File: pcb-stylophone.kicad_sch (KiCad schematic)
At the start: 2 parts, among them J1 Conn_01x02_Pin, U1 NA555P

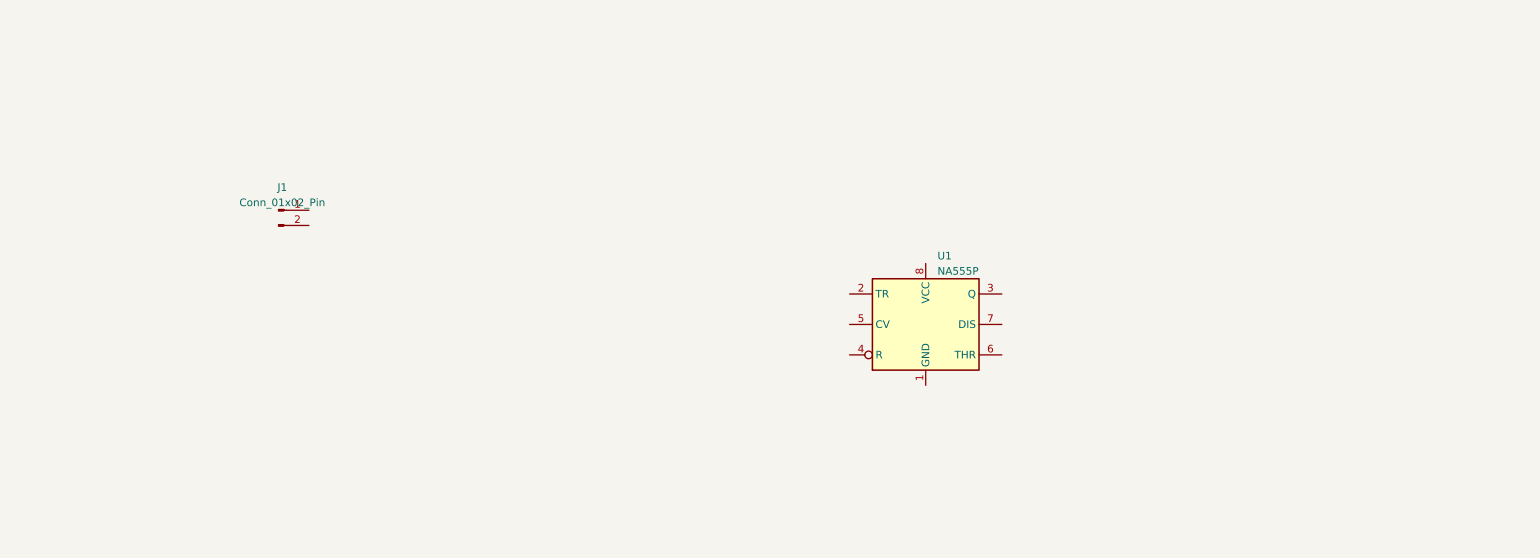
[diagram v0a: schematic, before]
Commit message: finalised v1
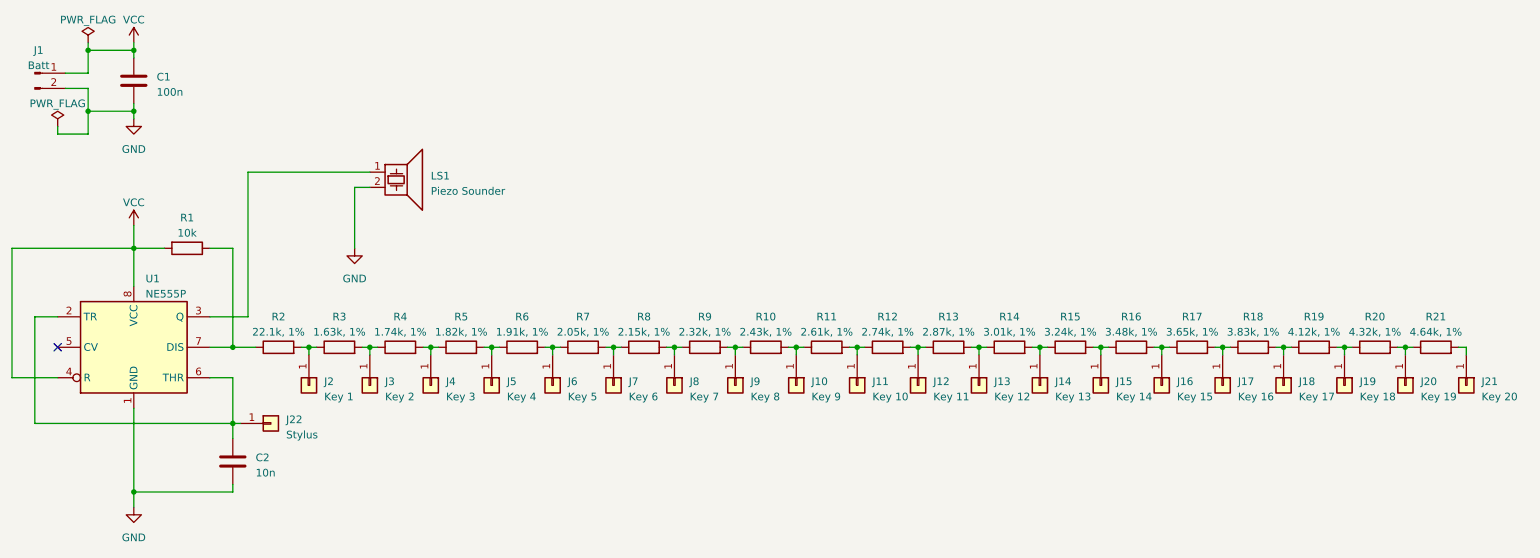
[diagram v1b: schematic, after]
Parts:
- removed U1: NA555P, Package_DIP:DIP-8_W7.62mm, symbol Timer:NA555P
- added C1: 100n, Capacitor_THT:C_Disc_D4.3mm_W1.9mm_P5.00mm, symbol Device:C
- added C2: 10n, Capacitor_THT:C_Disc_D4.3mm_W1.9mm_P5.00mm, symbol Device:C
- added J10: Key 9, TestPoint:TestPoint_Pad_1.0x1.0mm, symbol Connector_Generic:Conn_01x01
- added J11: Key 10, TestPoint:TestPoint_Pad_1.0x1.0mm, symbol Connector_Generic:Conn_01x01
- added J12: Key 11, TestPoint:TestPoint_Pad_1.0x1.0mm, symbol Connector_Generic:Conn_01x01
- added J13: Key 12, TestPoint:TestPoint_Pad_1.0x1.0mm, symbol Connector_Generic:Conn_01x01
- added J14: Key 13, TestPoint:TestPoint_Pad_1.0x1.0mm, symbol Connector_Generic:Conn_01x01
- added J15: Key 14, TestPoint:TestPoint_Pad_1.0x1.0mm, symbol Connector_Generic:Conn_01x01
- added J16: Key 15, TestPoint:TestPoint_Pad_1.0x1.0mm, symbol Connector_Generic:Conn_01x01
- added J17: Key 16, TestPoint:TestPoint_Pad_1.0x1.0mm, symbol Connector_Generic:Conn_01x01
- added J18: Key 17, TestPoint:TestPoint_Pad_1.0x1.0mm, symbol Connector_Generic:Conn_01x01
- added J19: Key 18, TestPoint:TestPoint_Pad_1.0x1.0mm, symbol Connector_Generic:Conn_01x01
- added J2: Key 1, TestPoint:TestPoint_Pad_1.0x1.0mm, symbol Connector_Generic:Conn_01x01
- added J20: Key 19, TestPoint:TestPoint_Pad_1.0x1.0mm, symbol Connector_Generic:Conn_01x01
- added J21: Key 20, TestPoint:TestPoint_Pad_1.0x1.0mm, symbol Connector_Generic:Conn_01x01
- added J22: Stylus, TestPoint:TestPoint_THTPad_D2.5mm_Drill1.2mm, symbol Connector_Generic:Conn_01x01
- added J3: Key 2, TestPoint:TestPoint_Pad_1.0x1.0mm, symbol Connector_Generic:Conn_01x01
- added J4: Key 3, TestPoint:TestPoint_Pad_1.0x1.0mm, symbol Connector_Generic:Conn_01x01
- added J5: Key 4, TestPoint:TestPoint_Pad_1.0x1.0mm, symbol Connector_Generic:Conn_01x01
- added J6: Key 5, TestPoint:TestPoint_Pad_1.0x1.0mm, symbol Connector_Generic:Conn_01x01
- added J7: Key 6, TestPoint:TestPoint_Pad_1.0x1.0mm, symbol Connector_Generic:Conn_01x01
- added J8: Key 7, TestPoint:TestPoint_Pad_1.0x1.0mm, symbol Connector_Generic:Conn_01x01
- added J9: Key 8, TestPoint:TestPoint_Pad_1.0x1.0mm, symbol Connector_Generic:Conn_01x01
- added LS1: Piezo Sounder, Buzzer_Beeper:Buzzer_D14mm_H7mm_P10mm, symbol Device:Speaker_Crystal
- added R1: 10k, Resistor_THT:R_Axial_DIN0207_L6.3mm_D2.5mm_P7.62mm_Horizontal, symbol Device:R
- added R10: 2.43k, 1%, Resistor_THT:R_Axial_DIN0207_L6.3mm_D2.5mm_P7.62mm_Horizontal, symbol Device:R
- added R11: 2.61k, 1%, Resistor_THT:R_Axial_DIN0207_L6.3mm_D2.5mm_P7.62mm_Horizontal, symbol Device:R
- added R12: 2.74k, 1%, Resistor_THT:R_Axial_DIN0207_L6.3mm_D2.5mm_P7.62mm_Horizontal, symbol Device:R
- added R13: 2.87k, 1%, Resistor_THT:R_Axial_DIN0207_L6.3mm_D2.5mm_P7.62mm_Horizontal, symbol Device:R
- added R14: 3.01k, 1%, Resistor_THT:R_Axial_DIN0207_L6.3mm_D2.5mm_P7.62mm_Horizontal, symbol Device:R
- added R15: 3.24k, 1%, Resistor_THT:R_Axial_DIN0207_L6.3mm_D2.5mm_P7.62mm_Horizontal, symbol Device:R
- added R16: 3.48k, 1%, Resistor_THT:R_Axial_DIN0207_L6.3mm_D2.5mm_P7.62mm_Horizontal, symbol Device:R
- added R17: 3.65k, 1%, Resistor_THT:R_Axial_DIN0207_L6.3mm_D2.5mm_P7.62mm_Horizontal, symbol Device:R
- added R18: 3.83k, 1%, Resistor_THT:R_Axial_DIN0207_L6.3mm_D2.5mm_P7.62mm_Horizontal, symbol Device:R
- added R19: 4.12k, 1%, Resistor_THT:R_Axial_DIN0207_L6.3mm_D2.5mm_P7.62mm_Horizontal, symbol Device:R
- added R2: 22.1k, 1%, Resistor_THT:R_Axial_DIN0207_L6.3mm_D2.5mm_P7.62mm_Horizontal, symbol Device:R
- added R20: 4.32k, 1%, Resistor_THT:R_Axial_DIN0207_L6.3mm_D2.5mm_P7.62mm_Horizontal, symbol Device:R
- added R21: 4.64k, 1%, Resistor_THT:R_Axial_DIN0207_L6.3mm_D2.5mm_P7.62mm_Horizontal, symbol Device:R
- added R3: 1.63k, 1%, Resistor_THT:R_Axial_DIN0207_L6.3mm_D2.5mm_P7.62mm_Horizontal, symbol Device:R
- added R4: 1.74k, 1%, Resistor_THT:R_Axial_DIN0207_L6.3mm_D2.5mm_P7.62mm_Horizontal, symbol Device:R
- added R5: 1.82k, 1%, Resistor_THT:R_Axial_DIN0207_L6.3mm_D2.5mm_P7.62mm_Horizontal, symbol Device:R
- added R6: 1.91k, 1%, Resistor_THT:R_Axial_DIN0207_L6.3mm_D2.5mm_P7.62mm_Horizontal, symbol Device:R
- added R7: 2.05k, 1%, Resistor_THT:R_Axial_DIN0207_L6.3mm_D2.5mm_P7.62mm_Horizontal, symbol Device:R
- added R8: 2.15k, 1%, Resistor_THT:R_Axial_DIN0207_L6.3mm_D2.5mm_P7.62mm_Horizontal, symbol Device:R
- added R9: 2.32k, 1%, Resistor_THT:R_Axial_DIN0207_L6.3mm_D2.5mm_P7.62mm_Horizontal, symbol Device:R
- added U1: NE555P, Package_DIP:DIP-8_W7.62mm, symbol Timer:NE555P
- J1: value Conn_01x02_Pin -> Batt; footprint (none) -> Connector_PinHeader_2.54mm:PinHeader_1x02_P2.54mm_Vertical
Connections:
- net VCC: now reaches J1.1 (Pin_1)
- net VCC: now also C1.1, R1.2, U1.4 (R), U1.8 (VCC)
- net GND: now reaches J1.2 (Pin_2)
- net GND: now also C1.2, C2.2, LS1.2, U1.1 (GND)
- new net: J11.1 (Pin_1), R11.2, R12.1
- new net: J12.1 (Pin_1), R12.2, R13.1
- new net: J10.1 (Pin_1), R10.2, R11.1
- new net: J21.1 (Pin_1), R21.2
- new net: R1.1, R2.1, U1.7 (DIS)
- new net: J9.1 (Pin_1), R10.1, R9.2
- new net: J17.1 (Pin_1), R17.2, R18.1
- new net: J18.1 (Pin_1), R18.2, R19.1
- new net: C2.1, J22.1 (Pin_1), U1.2 (TR), U1.6 (THR)
- new net: J15.1 (Pin_1), R15.2, R16.1
- new net: J16.1 (Pin_1), R16.2, R17.1
- new net: J20.1 (Pin_1), R20.2, R21.1
- new net: J7.1 (Pin_1), R7.2, R8.1
- new net: J8.1 (Pin_1), R8.2, R9.1
- new net: J13.1 (Pin_1), R13.2, R14.1
- new net: J14.1 (Pin_1), R14.2, R15.1
- new net: J5.1 (Pin_1), R5.2, R6.1
- new net: J4.1 (Pin_1), R4.2, R5.1
- new net: J6.1 (Pin_1), R6.2, R7.1
- new net: LS1.1, U1.3 (Q)
- new net: J19.1 (Pin_1), R19.2, R20.1
- new net: J3.1 (Pin_1), R3.2, R4.1
- new net: J2.1 (Pin_1), R2.2, R3.1
- no-connect marks 0 -> 1
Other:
- company: (none) -> The University of Manchester
- title: (none) -> PCB Stylophone

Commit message: stylophone v2 has bigger resistor soldering pads
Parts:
- R1, R10, R11, R12, R13, R14, R15, R16, R17, R18, R19, R2, R20, R21, R3, R4, R5, R6, R7, R8, R9: footprint Resistor_THT:R_Axial_DIN0207_L6.3mm_D2.5mm_P7.62mm_Horizontal -> Library:R_Axial_DIN0207_L6.3mm_D2.5mm_P10.16mm_Horizontal
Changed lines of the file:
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@@
       (effects (font (size 1.27 1.27)))
     )
-    (property "Footprint" "Resistor_THT:R_Axial_DIN0207_L6.3mm_D2.5mm_P7.62mm_Horizontal" (at 172.72 100.838 90)
+    (property "Footprint" "Library:R_Axial_DIN0207_L6.3mm_D2.5mm_P10.16mm_Horizontal" (at 172.72 100.838 90)
       (effects (font (size 1.27 1.27)) hide)
     )
@@
       (effects (font (size 1.27 1.27)))
     )
-    (property "Footprint" "Resistor_THT:R_Axial_DIN0207_L6.3mm_D2.5mm_P7.62mm_Horizontal" (at 55.88 80.772 90)
+    (property "Footprint" "Library:R_Axial_DIN0207_L6.3mm_D2.5mm_P10.16mm_Horizontal" (at 55.88 80.772 90)
       (effects (font (size 1.27 1.27)) hide)
     )
@@
       (effects (font (size 1.27 1.27)))
     )
-    (property "Footprint" "Resistor_THT:R_Axial_DIN0207_L6.3mm_D2.5mm_P7.62mm_Horizontal" (at 233.68 100.838 90)
+    (property "Footprint" "Library:R_Axial_DIN0207_L6.3mm_D2.5mm_P10.16mm_Horizontal" (at 233.68 100.838 90)
       (effects (font (size 1.27 1.27)) hide)
     )
@@
       (effects (font (size 1.27 1.27)))
     )
-    (property "Footprint" "Resistor_THT:R_Axial_DIN0207_L6.3mm_D2.5mm_P7.62mm_Horizontal" (at 213.36 100.838 90)
+    (property "Footprint" "Library:R_Axial_DIN0207_L6.3mm_D2.5mm_P10.16mm_Horizontal" (at 213.36 100.838 90)
       (effects (font (size 1.27 1.27)) hide)
     )
@@
       (effects (font (size 1.27 1.27)))
     )
-    (property "Footprint" "Resistor_THT:R_Axial_DIN0207_L6.3mm_D2.5mm_P7.62mm_Horizontal" (at 264.16 100.838 90)
+    (property "Footprint" "Library:R_Axial_DIN0207_L6.3mm_D2.5mm_P10.16mm_Horizontal" (at 264.16 100.838 90)
       (effects (font (size 1.27 1.27)) hide)
     )
@@
       (effects (font (size 1.27 1.27)))
     )
-    (property "Footprint" "Resistor_THT:R_Axial_DIN0207_L6.3mm_D2.5mm_P7.62mm_Horizontal" (at 132.08 100.838 90)
+    (property "Footprint" "Library:R_Axial_DIN0207_L6.3mm_D2.5mm_P10.16mm_Horizontal" (at 132.08 100.838 90)
       (effects (font (size 1.27 1.27)) hide)
     )
@@
       (effects (font (size 1.27 1.27)))
     )
-    (property "Footprint" "Resistor_THT:R_Axial_DIN0207_L6.3mm_D2.5mm_P7.62mm_Horizontal" (at 193.04 100.838 90)
+    (property "Footprint" "Library:R_Axial_DIN0207_L6.3mm_D2.5mm_P10.16mm_Horizontal" (at 193.04 100.838 90)
       (effects (font (size 1.27 1.27)) hide)
     )
@@
       (effects (font (size 1.27 1.27)))
     )
-    (property "Footprint" "Resistor_THT:R_Axial_DIN0207_L6.3mm_D2.5mm_P7.62mm_Horizontal" (at 142.24 100.838 90)
+    (property "Footprint" "Library:R_Axial_DIN0207_L6.3mm_D2.5mm_P10.16mm_Horizontal" (at 142.24 100.838 90)
       (effects (font (size 1.27 1.27)) hide)
     )
@@
       (effects (font (size 1.27 1.27)))
     )
-    (property "Footprint" "Resistor_THT:R_Axial_DIN0207_L6.3mm_D2.5mm_P7.62mm_Horizontal" (at 223.52 100.838 90)
+    (property "Footprint" "Library:R_Axial_DIN0207_L6.3mm_D2.5mm_P10.16mm_Horizontal" (at 223.52 100.838 90)
       (effects (font (size 1.27 1.27)) hide)
     )
@@
       (effects (font (size 1.27 1.27)))
     )
-    (property "Footprint" "Resistor_THT:R_Axial_DIN0207_L6.3mm_D2.5mm_P7.62mm_Horizontal" (at 152.4 100.838 90)
+    (property "Footprint" "Library:R_Axial_DIN0207_L6.3mm_D2.5mm_P10.16mm_Horizontal" (at 152.4 100.838 90)
       (effects (font (size 1.27 1.27)) hide)
     )
@@
       (effects (font (size 1.27 1.27)))
     )
-    (property "Footprint" "Resistor_THT:R_Axial_DIN0207_L6.3mm_D2.5mm_P7.62mm_Horizontal" (at 243.84 100.838 90)
+    (property "Footprint" "Library:R_Axial_DIN0207_L6.3mm_D2.5mm_P10.16mm_Horizontal" (at 243.84 100.838 90)
       (effects (font (size 1.27 1.27)) hide)
     )
@@
       (effects (font (size 1.27 1.27)))
     )
-    (property "Footprint" "Resistor_THT:R_Axial_DIN0207_L6.3mm_D2.5mm_P7.62mm_Horizontal" (at 182.88 100.838 90)
+    (property "Footprint" "Library:R_Axial_DIN0207_L6.3mm_D2.5mm_P10.16mm_Horizontal" (at 182.88 100.838 90)
       (effects (font (size 1.27 1.27)) hide)
     )
@@
       (effects (font (size 1.27 1.27)))
     )
-    (property "Footprint" "Resistor_THT:R_Axial_DIN0207_L6.3mm_D2.5mm_P7.62mm_Horizontal" (at 81.28 100.838 90)
+    (property "Footprint" "Library:R_Axial_DIN0207_L6.3mm_D2.5mm_P10.16mm_Horizontal" (at 81.28 100.838 90)
       (effects (font (size 1.27 1.27)) hide)
     )
@@
       (effects (font (size 1.27 1.27)))
     )
-    (property "Footprint" "Resistor_THT:R_Axial_DIN0207_L6.3mm_D2.5mm_P7.62mm_Horizontal" (at 121.92 100.838 90)
+    (property "Footprint" "Library:R_Axial_DIN0207_L6.3mm_D2.5mm_P10.16mm_Horizontal" (at 121.92 100.838 90)
       (effects (font (size 1.27 1.27)) hide)
     )
@@
       (effects (font (size 1.27 1.27)))
     )
-    (property "Footprint" "Resistor_THT:R_Axial_DIN0207_L6.3mm_D2.5mm_P7.62mm_Horizontal" (at 162.56 100.838 90)
+    (property "Footprint" "Library:R_Axial_DIN0207_L6.3mm_D2.5mm_P10.16mm_Horizontal" (at 162.56 100.838 90)
       (effects (font (size 1.27 1.27)) hide)
     )
@@
       (effects (font (size 1.27 1.27)))
     )
-    (property "Footprint" "Resistor_THT:R_Axial_DIN0207_L6.3mm_D2.5mm_P7.62mm_Horizontal" (at 91.44 100.838 90)
+    (property "Footprint" "Library:R_Axial_DIN0207_L6.3mm_D2.5mm_P10.16mm_Horizontal" (at 91.44 100.838 90)
       (effects (font (size 1.27 1.27)) hide)
     )
@@
       (effects (font (size 1.27 1.27)))
     )
-    (property "Footprint" "Resistor_THT:R_Axial_DIN0207_L6.3mm_D2.5mm_P7.62mm_Horizontal" (at 254 100.838 90)
+    (property "Footprint" "Library:R_Axial_DIN0207_L6.3mm_D2.5mm_P10.16mm_Horizontal" (at 254 100.838 90)
       (effects (font (size 1.27 1.27)) hide)
     )
@@
       (effects (font (size 1.27 1.27)))
     )
-    (property "Footprint" "Resistor_THT:R_Axial_DIN0207_L6.3mm_D2.5mm_P7.62mm_Horizontal" (at 101.6 100.838 90)
+    (property "Footprint" "Library:R_Axial_DIN0207_L6.3mm_D2.5mm_P10.16mm_Horizontal" (at 101.6 100.838 90)
       (effects (font (size 1.27 1.27)) hide)
     )
@@
       (effects (font (size 1.27 1.27)))
     )
-    (property "Footprint" "Resistor_THT:R_Axial_DIN0207_L6.3mm_D2.5mm_P7.62mm_Horizontal" (at 111.76 100.838 90)
+    (property "Footprint" "Library:R_Axial_DIN0207_L6.3mm_D2.5mm_P10.16mm_Horizontal" (at 111.76 100.838 90)
       (effects (font (size 1.27 1.27)) hide)
     )
@@
       (effects (font (size 1.27 1.27)))
     )
-    (property "Footprint" "Resistor_THT:R_Axial_DIN0207_L6.3mm_D2.5mm_P7.62mm_Horizontal" (at 71.12 100.838 90)
+    (property "Footprint" "Library:R_Axial_DIN0207_L6.3mm_D2.5mm_P10.16mm_Horizontal" (at 71.12 100.838 90)
       (effects (font (size 1.27 1.27)) hide)
     )
@@
       (effects (font (size 1.27 1.27)))
     )
-    (property "Footprint" "Resistor_THT:R_Axial_DIN0207_L6.3mm_D2.5mm_P7.62mm_Horizontal" (at 203.2 100.838 90)
-      (effects (font (size 1.27 1.27)) hide)
-    )
+    (property "Footprint" "Library:R_Axial_DIN0207_L6.3mm_D2.5mm_P10.16mm_Horizontal" (at 203.2 100.838 90)
+      (effects (font (size 1.27 1.27)) hide)
+    )
